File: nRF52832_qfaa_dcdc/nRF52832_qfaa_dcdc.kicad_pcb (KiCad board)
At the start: 2 copper layers, 52.1 x 34.3 mm, 22 parts, among them SW1 SW_Push, U1 NRF52832, X1 32MHz, X2 32.768kHz

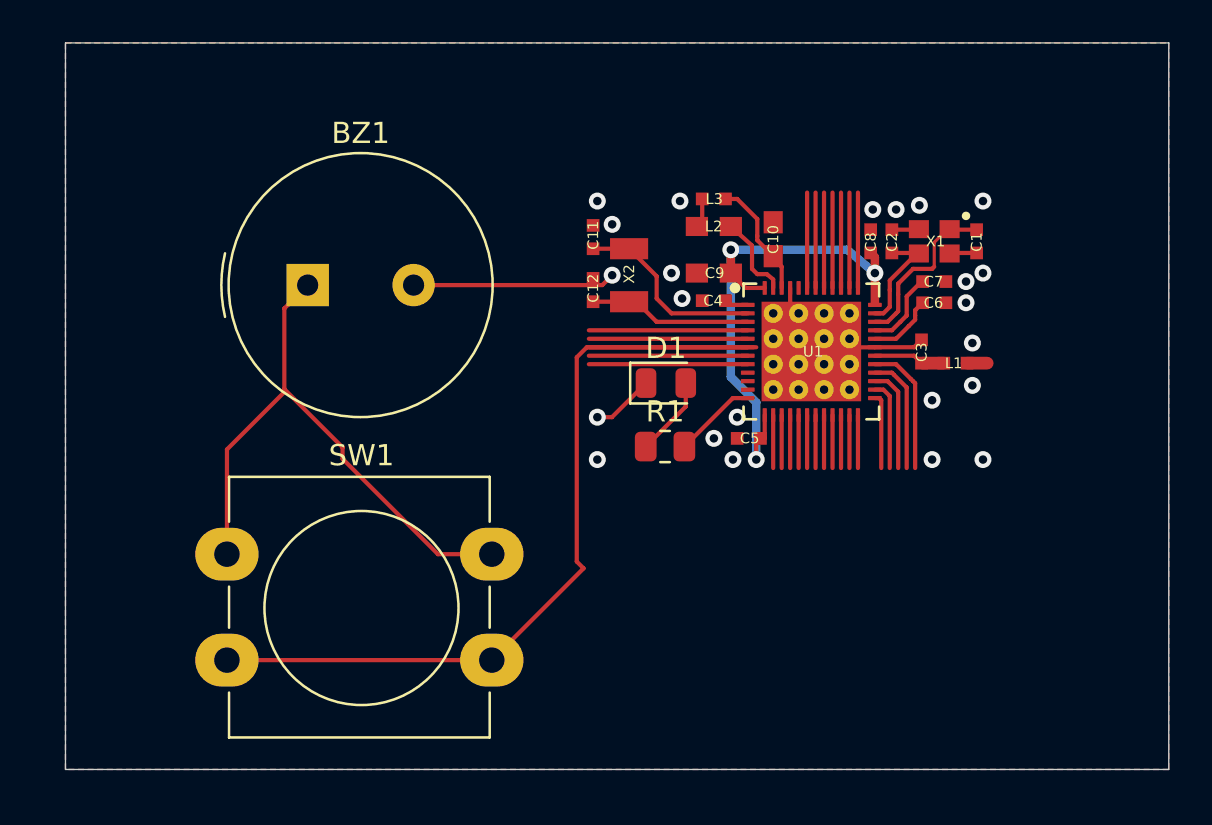
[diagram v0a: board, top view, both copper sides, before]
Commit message: commit changement elec
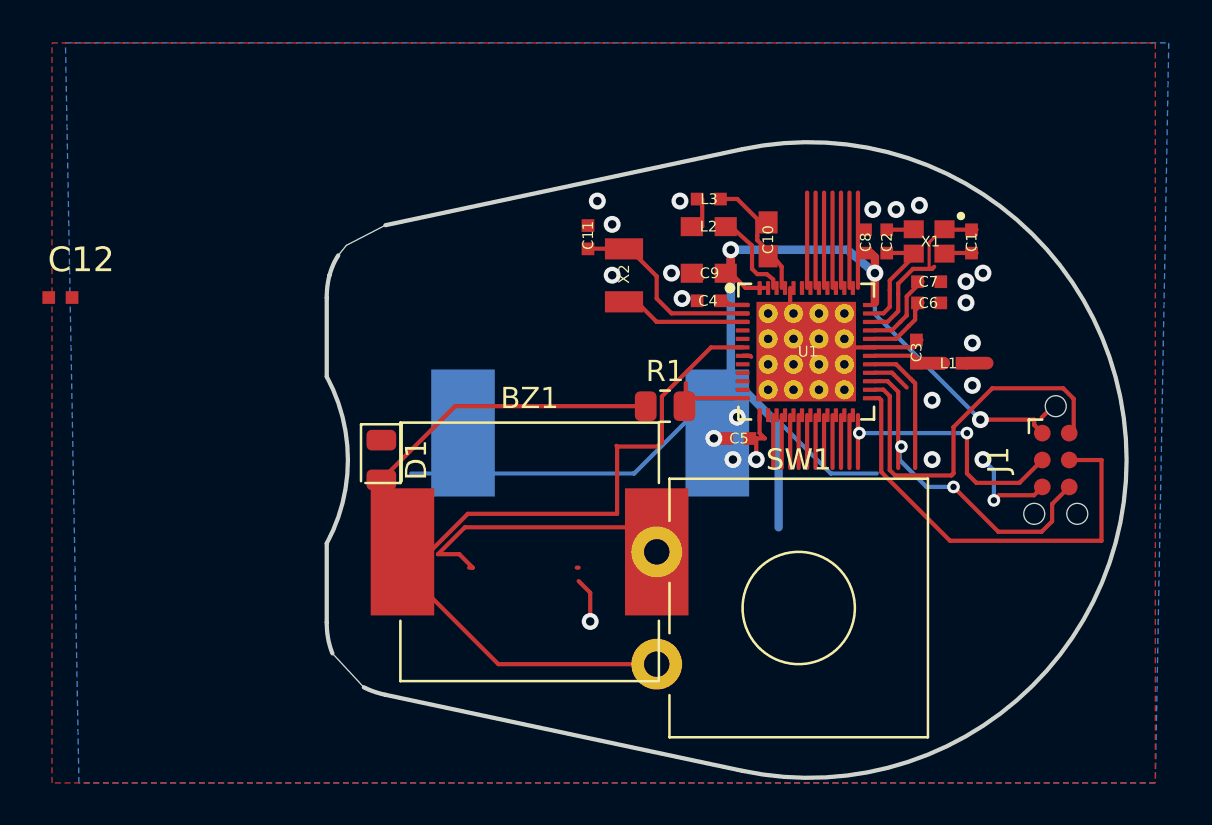
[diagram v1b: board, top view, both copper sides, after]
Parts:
- added BT1: Battery_Cell, Buzzer_Beeper:Buzzer_Mallory_AST1240MLQ, B.Cu at (139.1, 109.9)
- added J1: Conn_ARM_SWD_TagConnect_TC2030-NL, Connector:Tag-Connect_TC2030-IDC-NL_2x03_P1.27mm_Vertical, F.Cu at (161.0, 111.1)
- BZ1: footprint Buzzer_Beeper:Buzzer_TDK_PS1240P02BT_D12.2mm_H6.5mm -> Buzzer_Beeper:Buzzer_Mallory_AST1240MLQ
- SW1: footprint Button_Switch_THT:SW_PUSH-12mm_Wuerth-430476085716 -> Button_Switch_THT:SW_CW_GPTS203211B
- moved C12 25.1 mm to (114.1, 103.5), turned to 0 degrees
- moved SW1 20.3 mm to (142.2, 115.5)
- moved BZ1 16.4 mm to (136.2, 115.5)
- moved D1 13.9 mm to (129.2, 111.1), turned to -90 degrees
- moved R1 1.91 mm to (142.6, 108.6)
- moved C5 0.50 mm to (146.1, 110.1)
- moved C4 0.24 mm to (144.7, 103.6)
- moved C9 0.24 mm to (144.7, 102.3)
- moved L2 0.24 mm to (144.7, 100.1)
- moved L3 0.24 mm to (144.7, 98.8)
- moved U1 0.24 mm to (149.3, 106.0)
- moved X2 0.24 mm to (140.7, 102.4)
- moved C1 0.24 mm to (157.1, 100.8)
- moved C10 0.24 mm to (147.5, 100.7)
- moved C11 0.24 mm to (139.0, 100.6)
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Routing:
- net VCC: track 25.6 -> 68.9 mm, vias 3 -> 4
- net /SWDCLK: track 3.54 -> 20.8 mm
- net /SWDIO: track 4.22 -> 18.0 mm
- net /P0.21/RESET: track 2.50 -> 16.2 mm, vias 0 -> 2
- net Net-(BZ1--): track 27.6 -> 14.1 mm
- net /P0.22: track 4.91 -> 16.3 mm, vias 0 -> 2
- net Net-(D1-A): track 3.78 -> 13.9 mm
- net /P0.04: track 44.9 -> 37.3 mm
- net /P0.06: track 7.50 -> 0.00 mm
- net /P0.03: track 7.50 -> 0.00 mm
- net /P0.02: track 7.50 -> 0.00 mm
- net /P0.05: track 7.50 -> 0.66 mm
- net /P0.31: track 4.50 -> 0.00 mm
- net /P0.25: track 4.50 -> 9.00 mm
- net Net-(U1-DCC@47): track 4.04 -> 0.00 mm
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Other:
- board size 52.1 x 34.3 mm -> 37.8 x 30 mm
